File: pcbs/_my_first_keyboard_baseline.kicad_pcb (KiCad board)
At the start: 2 copper layers, 135.9 x 108 mm, 74 parts

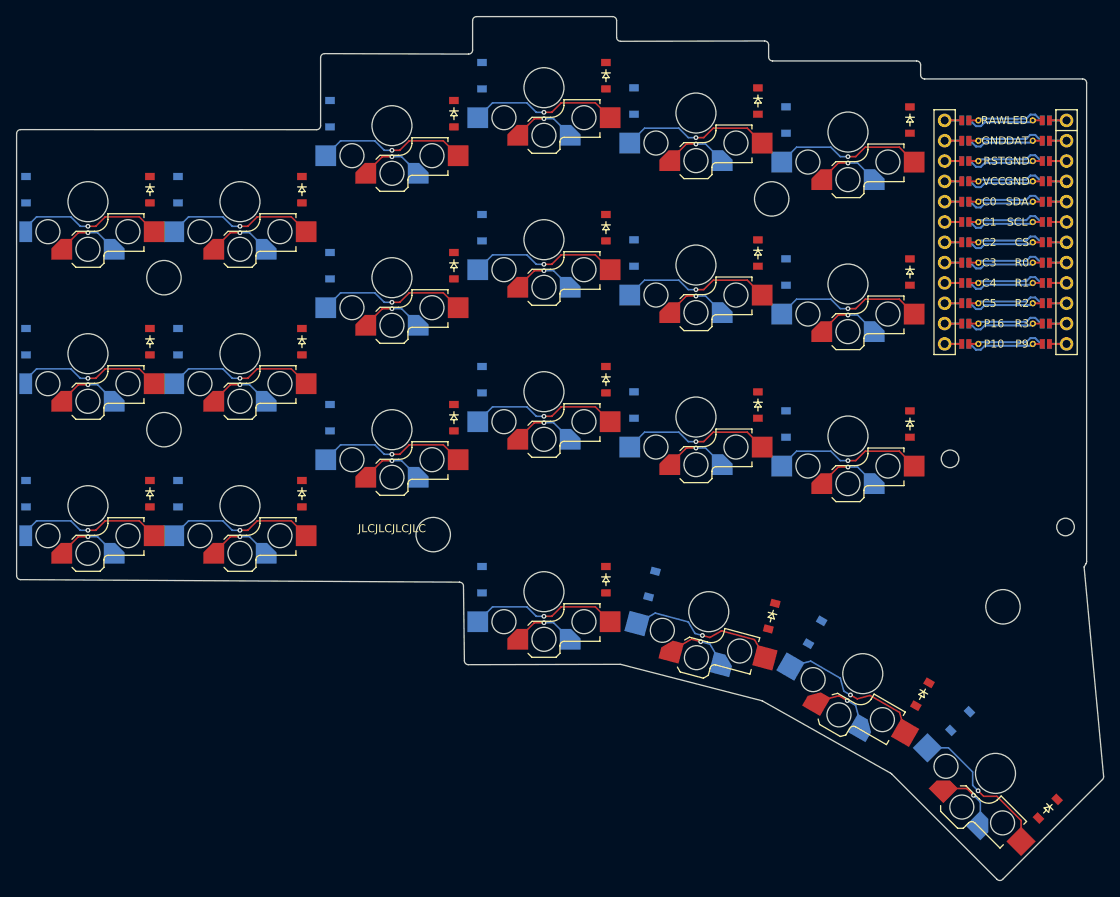
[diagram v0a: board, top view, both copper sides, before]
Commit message: v1
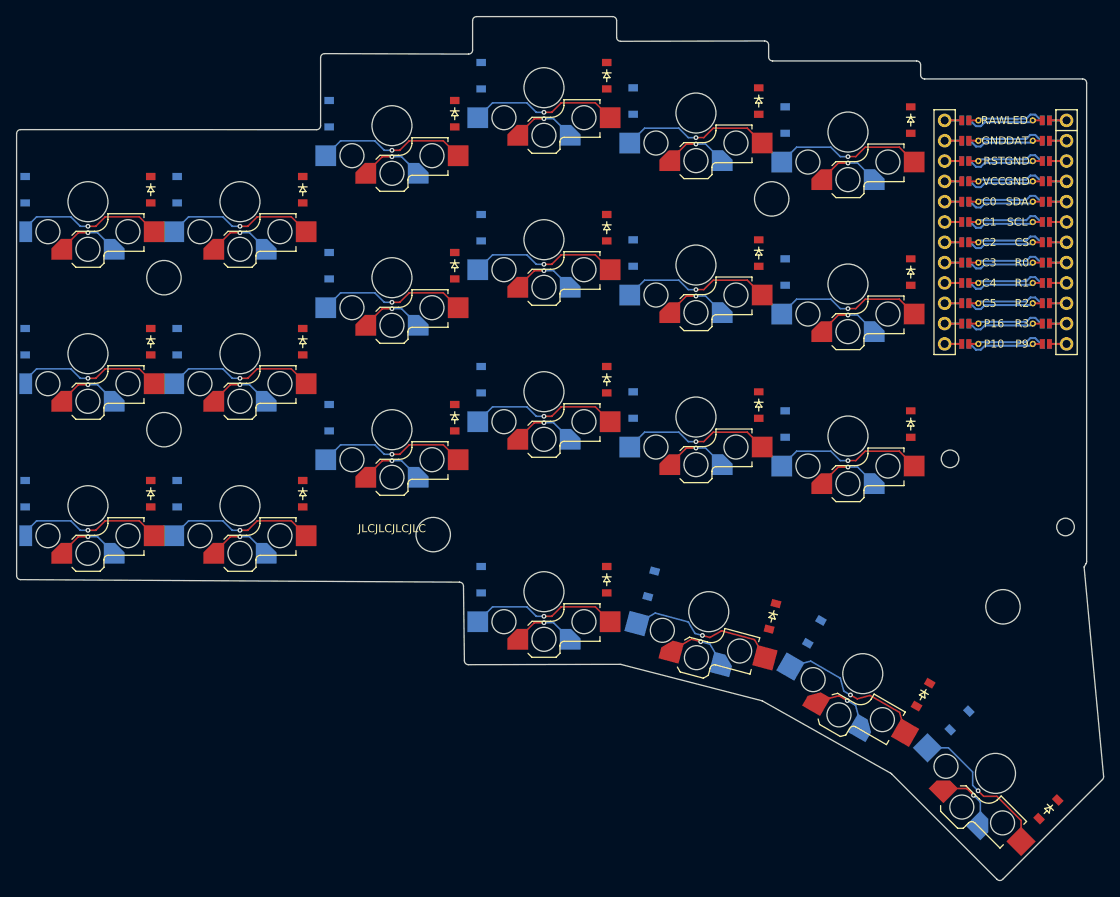
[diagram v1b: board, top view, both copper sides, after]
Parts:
- moved D22 0.10 mm to (209.0, 126.9)
- moved D44 0.10 mm to (220.1, 138.0)
- moved D42 0.10 mm to (185.6, 113.8)
- moved D20 0.10 mm to (170.4, 109.8)
- moved D1 0.10 mm to (92.2, 98.5)
- moved D10 0.10 mm to (149.2, 84.2)
- moved D11 0.10 mm to (149.2, 65.2)
- moved D12 0.10 mm to (149.2, 46.2)
- moved D13 0.10 mm to (168.2, 87.4)
- moved D14 0.10 mm to (168.2, 68.4)
- moved D15 0.10 mm to (168.2, 49.4)
- moved D16 0.10 mm to (187.2, 89.8)
- moved D17 0.10 mm to (187.2, 70.8)
- moved D18 0.10 mm to (187.2, 51.8)
- moved D19 0.10 mm to (149.2, 109.2)
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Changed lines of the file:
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@@
   (title_block
     (title "_my_first_keyboard_baseline")
-    (date "2026-05-17")
+    (date "2026-05-21")
     (rev "0.1")
     (company "Unknown")
@@
     (footprint "ceoloide:diode_tht_sod123"
         (layer "B.Cu")
-        (at 92.25 98.5 -90)
+        (at 92.15 98.5 -90)
         (property "Reference" "D1"
             (at 0 0 -90)
@@
     (footprint "ceoloide:diode_tht_sod123"
         (layer "B.Cu")
-        (at 92.25 79.5 -90)
+        (at 92.15 79.5 -90)
         (property "Reference" "D2"
             (at 0 0 -90)
@@
     (footprint "ceoloide:diode_tht_sod123"
         (layer "B.Cu")
-        (at 92.25 60.5 -90)
+        (at 92.15 60.5 -90)
         (property "Reference" "D3"
             (at 0 0 -90)
@@
     (footprint "ceoloide:diode_tht_sod123"
         (layer "B.Cu")
-        (at 111.25 98.5 -90)
+        (at 111.15 98.5 -90)
         (property "Reference" "D4"
             (at 0 0 -90)
@@
     (footprint "ceoloide:diode_tht_sod123"
         (layer "B.Cu")
-        (at 111.25 79.5 -90)
+        (at 111.15 79.5 -90)
         (property "Reference" "D5"
             (at 0 0 -90)
@@
     (footprint "ceoloide:diode_tht_sod123"
         (layer "B.Cu")
-        (at 111.25 60.5 -90)
+        (at 111.15 60.5 -90)
         (property "Reference" "D6"
             (at 0 0 -90)
@@
     (footprint "ceoloide:diode_tht_sod123"
         (layer "B.Cu")
-        (at 130.25 89 -90)
+        (at 130.15 89 -90)
         (property "Reference" "D7"
             (at 0 0 -90)
@@
     (footprint "ceoloide:diode_tht_sod123"
         (layer "B.Cu")
-        (at 130.25 70 -90)
+        (at 130.15 70 -90)
         (property "Reference" "D8"
             (at 0 0 -90)
@@
     (footprint "ceoloide:diode_tht_sod123"
         (layer "B.Cu")
-        (at 130.25 51 -90)
+        (at 130.15 51 -90)
         (property "Reference" "D9"
             (at 0 0 -90)
@@
     (footprint "ceoloide:diode_tht_sod123"
         (layer "B.Cu")
-        (at 149.25 84.25 -90)
+        (at 149.15 84.25 -90)
         (property "Reference" "D10"
             (at 0 0 -90)
@@
     (footprint "ceoloide:diode_tht_sod123"
         (layer "B.Cu")
-        (at 149.25 65.25 -90)
+        (at 149.15 65.25 -90)
         (property "Reference" "D11"
             (at 0 0 -90)
@@
     (footprint "ceoloide:diode_tht_sod123"
         (layer "B.Cu")
-        (at 149.25 46.25 -90)
+        (at 149.15 46.25 -90)
         (property "Reference" "D12"
             (at 0 0 -90)
@@
     (footprint "ceoloide:diode_tht_sod123"
         (layer "B.Cu")
-        (at 168.25 87.41666670000001 -90)
+        (at 168.15 87.41666670000001 -90)
         (property "Reference" "D13"
             (at 0 0 -90)
@@
     (footprint "ceoloide:diode_tht_sod123"
         (layer "B.Cu")
-        (at 168.25 68.41666670000001 -90)
+        (at 168.15 68.41666670000001 -90)
         (property "Reference" "D14"
             (at 0 0 -90)
@@
     (footprint "ceoloide:diode_tht_sod123"
         (layer "B.Cu")
-        (at 168.25 49.41666670000001 -90)
+        (at 168.15 49.41666670000001 -90)
         (property "Reference" "D15"
             (at 0 0 -90)
@@
     (footprint "ceoloide:diode_tht_sod123"
         (layer "B.Cu")
-        (at 187.25 89.79166670000001 -90)
+        (at 187.15 89.79166670000001 -90)
         (property "Reference" "D16"
             (at 0 0 -90)
@@
     (footprint "ceoloide:diode_tht_sod123"
         (layer "B.Cu")
-        (at 187.25 70.79166670000001 -90)
+        (at 187.15 70.79166670000001 -90)
         (property "Reference" "D17"
             (at 0 0 -90)
@@
     (footprint "ceoloide:diode_tht_sod123"
         (layer "B.Cu")
-        (at 187.25 51.79166670000001 -90)
+        (at 187.15 51.79166670000001 -90)
         (property "Reference" "D18"
             (at 0 0 -90)
@@
     (footprint "ceoloide:diode_tht_sod123"
         (layer "B.Cu")
-        (at 149.25 109.25 -90)
+        (at 149.15 109.25 -90)
         (property "Reference" "D19"
             (at 0 0 -90)
@@
     (footprint "ceoloide:diode_tht_sod123"
         (layer "B.Cu")
-        (at 170.5023034 109.7952637 -105)
+        (at 170.4057108 109.7693818 -105)
         (property "Reference" "D20"
             (at 0 0 -105)
@@
     (footprint "ceoloide:diode_tht_sod123"
         (layer "B.Cu")
-        (at 190.8893275 115.82244879999999 -120)
+        (at 190.802725 115.77244879999999 -120)
         (property "Reference" "D21"
             (at 0 0 -120)
@@
     (footprint "ceoloide:diode_tht_sod123"
         (layer "B.Cu")
-        (at 209.0217303 126.9208127 -135)
+        (at 208.9510196 126.85010199999999 -135)
         (property "Reference" "D22"
             (at 0 0 -135)
@@
     (footprint "ceoloide:diode_tht_sod123"
         (layer "F.Cu")
-        (at 107.75 98.5 -90)
+        (at 107.85 98.5 -90)
         (property "Reference" "D23"
             (at 0 0 -90)
@@
     (footprint "ceoloide:diode_tht_sod123"
         (layer "F.Cu")
-        (at 107.75 79.5 -90)
+        (at 107.85 79.5 -90)
         (property "Reference" "D24"
             (at 0 0 -90)
@@
     (footprint "ceoloide:diode_tht_sod123"
         (layer "F.Cu")
-        (at 107.75 60.5 -90)
+        (at 107.85 60.5 -90)
         (property "Reference" "D25"
             (at 0 0 -90)
@@
     (footprint "ceoloide:diode_tht_sod123"
         (layer "F.Cu")
-        (at 126.75 98.5 -90)
+        (at 126.85 98.5 -90)
         (property "Reference" "D26"
             (at 0 0 -90)
@@
     (footprint "ceoloide:diode_tht_sod123"
         (layer "F.Cu")
-        (at 126.75 79.5 -90)
+        (at 126.85 79.5 -90)
         (property "Reference" "D27"
             (at 0 0 -90)
@@
     (footprint "ceoloide:diode_tht_sod123"
         (layer "F.Cu")
-        (at 126.75 60.5 -90)
+        (at 126.85 60.5 -90)
         (property "Reference" "D28"
             (at 0 0 -90)
@@
     (footprint "ceoloide:diode_tht_sod123"
         (layer "F.Cu")
-        (at 145.75 89 -90)
+        (at 145.85 89 -90)
         (property "Reference" "D29"
             (at 0 0 -90)
@@
     (footprint "ceoloide:diode_tht_sod123"
         (layer "F.Cu")
-        (at 145.75 70 -90)
+        (at 145.85 70 -90)
         (property "Reference" "D30"
             (at 0 0 -90)
@@
     (footprint "ceoloide:diode_tht_sod123"
         (layer "F.Cu")
-        (at 145.75 51 -90)
+        (at 145.85 51 -90)
         (property "Reference" "D31"
             (at 0 0 -90)
@@
     (footprint "ceoloide:diode_tht_sod123"
         (layer "F.Cu")
-        (at 164.75 84.25 -90)
+        (at 164.85 84.25 -90)
         (property "Reference" "D32"
             (at 0 0 -90)
@@
     (footprint "ceoloide:diode_tht_sod123"
         (layer "F.Cu")
-        (at 164.75 65.25 -90)
+        (at 164.85 65.25 -90)
         (property "Reference" "D33"
             (at 0 0 -90)
@@
     (footprint "ceoloide:diode_tht_sod123"
         (layer "F.Cu")
-        (at 164.75 46.25 -90)
+        (at 164.85 46.25 -90)
         (property "Reference" "D34"
             (at 0 0 -90)
@@
     (footprint "ceoloide:diode_tht_sod123"
         (layer "F.Cu")
-        (at 183.75 87.41666670000001 -90)
+        (at 183.85 87.41666670000001 -90)
         (property "Reference" "D35"
             (at 0 0 -90)
@@
     (footprint "ceoloide:diode_tht_sod123"
         (layer "F.Cu")
-        (at 183.75 68.41666670000001 -90)
+        (at 183.85 68.41666670000001 -90)
         (property "Reference" "D36"
             (at 0 0 -90)
@@
     (footprint "ceoloide:diode_tht_sod123"
         (layer "F.Cu")
-        (at 183.75 49.41666670000001 -90)
+        (at 183.85 49.41666670000001 -90)
         (property "Reference" "D37"
             (at 0 0 -90)
@@
     (footprint "ceoloide:diode_tht_sod123"
         (layer "F.Cu")
-        (at 202.75 89.79166670000001 -90)
+        (at 202.85 89.79166670000001 -90)
         (property "Reference" "D38"
             (at 0 0 -90)
@@
     (footprint "ceoloide:diode_tht_sod123"
         (layer "F.Cu")
-        (at 202.75 70.79166670000001 -90)
+        (at 202.85 70.79166670000001 -90)
         (property "Reference" "D39"
             (at 0 0 -90)
@@
     (footprint "ceoloide:diode_tht_sod123"
         (layer "F.Cu")
-        (at 202.75 51.79166670000001 -90)
+        (at 202.85 51.79166670000001 -90)
         (property "Reference" "D40"
             (at 0 0 -90)
@@
     (footprint "ceoloide:diode_tht_sod123"
         (layer "F.Cu")
-        (at 164.75 109.25 -90)
+        (at 164.85 109.25 -90)
         (property "Reference" "D41"
             (at 0 0 -90)
@@
     (footprint "ceoloide:diode_tht_sod123"
         (layer "F.Cu")
-        (at 185.4741537 113.8069589 -105)
+        (at 185.5707463 113.8328408 -105)
         (property "Reference" "D42"
             (at 0 0 -105)
@@
     (footprint "ceoloide:diode_tht_sod123"
         (layer "F.Cu")
-        (at 204.3127213 123.57244879999999 -120)
+        (at 204.3993238 123.6224488 -120)
         (property "Reference" "D43"
             (at 0 0 -120)
@@
     (footprint "ceoloide:diode_tht_sod123"
         (layer "F.Cu")
-        (at 219.98188539999998 137.8809678 -135)
+        (at 220.0525961 137.95167849999999 -135)
         (property "Reference" "D44"
             (at 0 0 -135)
